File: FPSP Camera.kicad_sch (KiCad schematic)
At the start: 0 parts

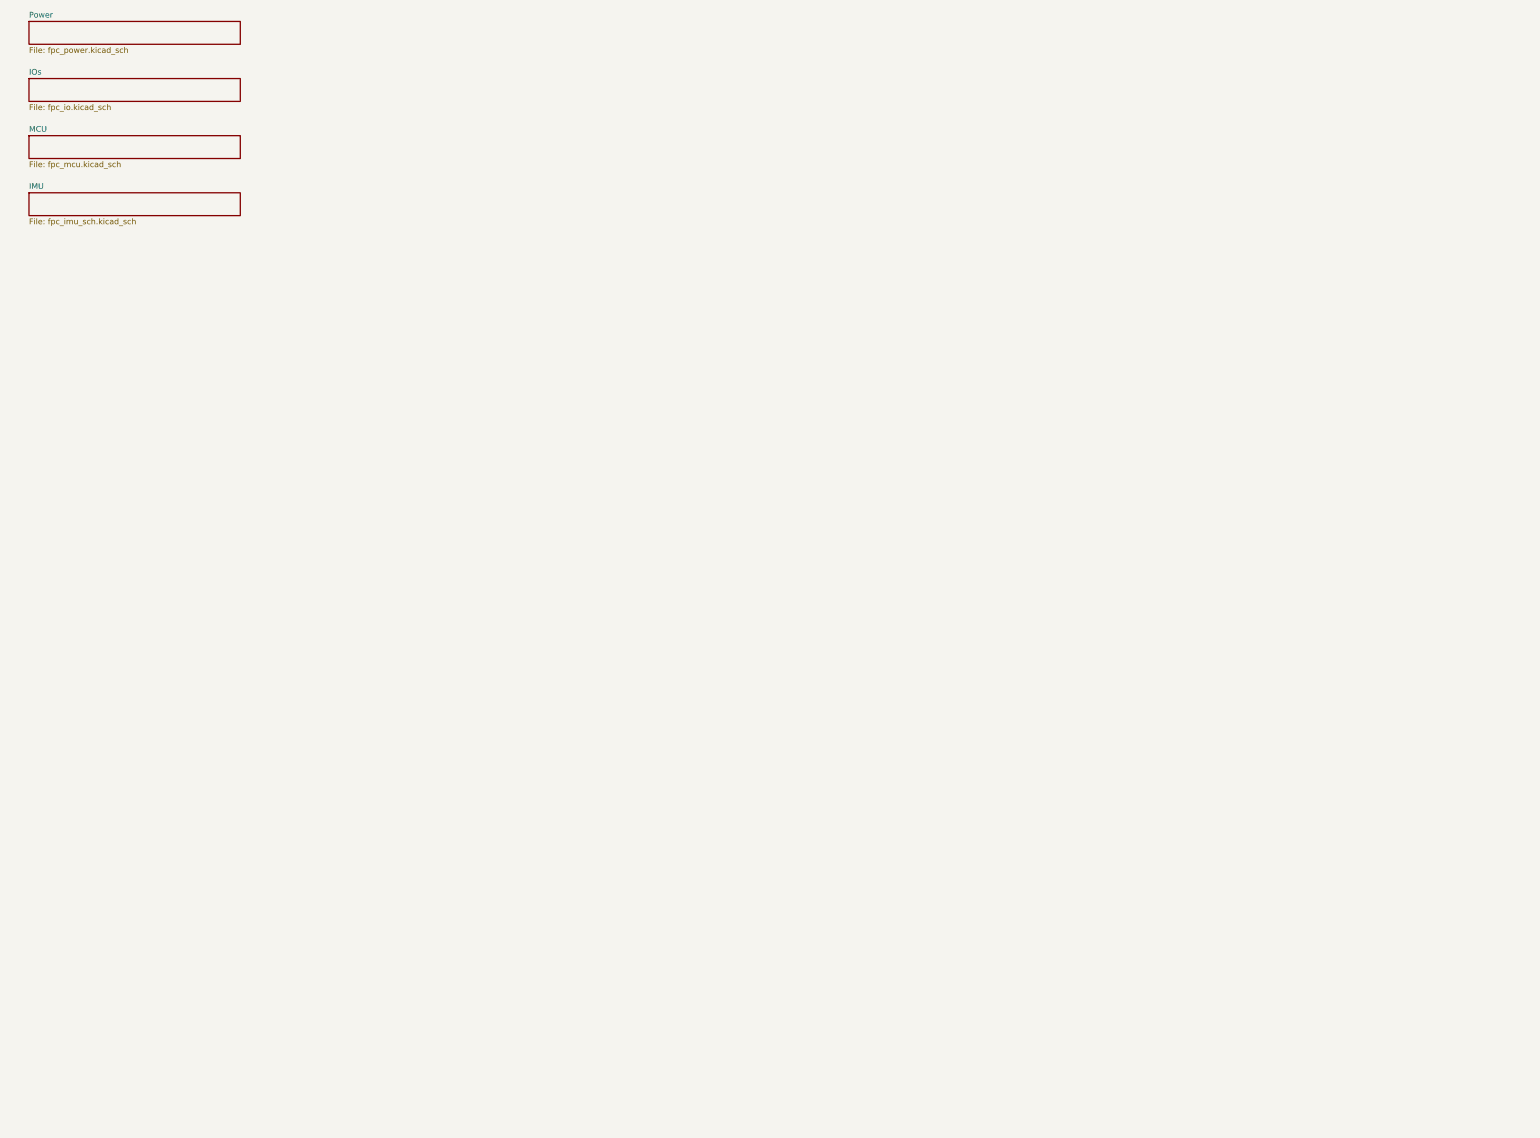
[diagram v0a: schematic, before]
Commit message: Cleanup
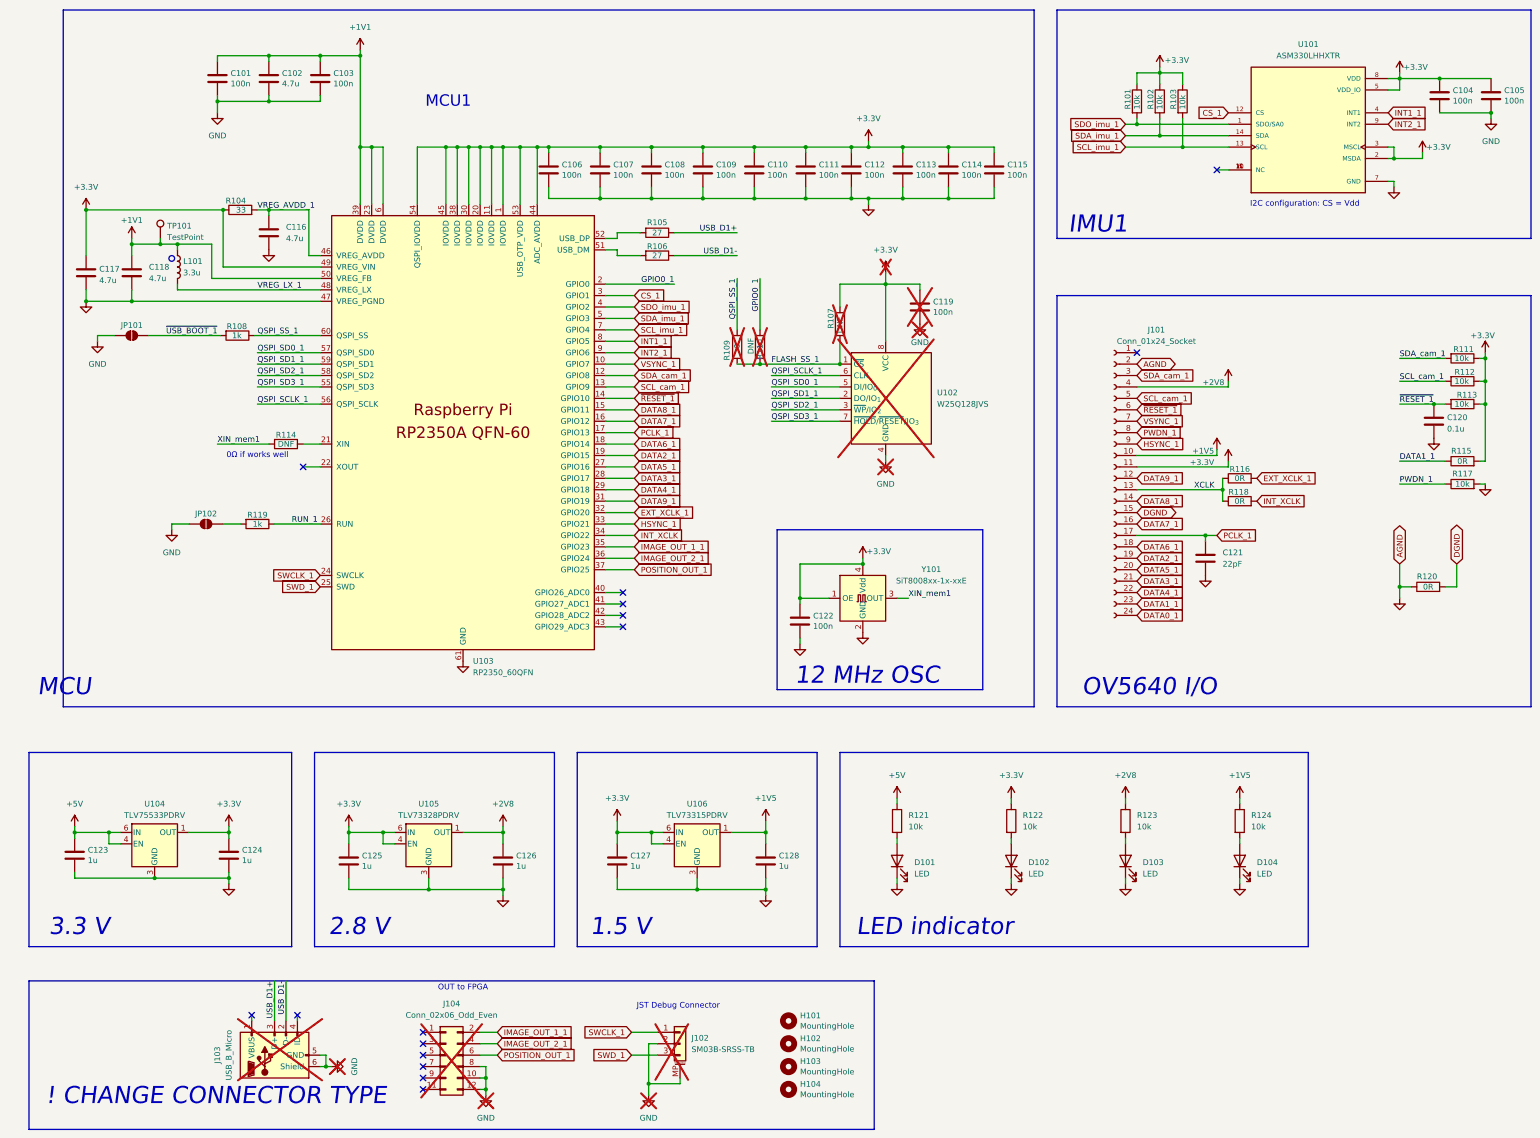
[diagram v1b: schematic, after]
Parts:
- added C101, C103, C104, C105, C106, C107, C108, C109, C110, C111, C112, C113, C114, C115, C119, C122: 100n, Capacitor_SMD:C_0603_1608Metric_Pad1.08x0.95mm_HandSolder, symbol Device:C
- added C102, C116, C117, C118: 4.7u, Capacitor_SMD:C_0603_1608Metric_Pad1.08x0.95mm_HandSolder, symbol Device:C
- added C120: 0.1u, Capacitor_SMD:C_0603_1608Metric_Pad1.08x0.95mm_HandSolder, symbol Device:C
- added C121: 22pF, Capacitor_SMD:C_0603_1608Metric_Pad1.08x0.95mm_HandSolder, symbol Device:C
- added C123, C124, C125, C126, C127, C128: 1u, Capacitor_SMD:C_0603_1608Metric_Pad1.08x0.95mm_HandSolder, symbol Device:C
- added D101, D102, D103, D104: LED, Diode_SMD:D_0603_1608Metric, symbol Device:LED
- added H101, H102, H103, H104: MountingHole, MountingHole:MountingHole_2.7mm_M2.5, symbol Mechanical:MountingHole
- added J101: Conn_01x24_Socket, Connector_FFC-FPC:TE_2-84952-4_1x24-1MP_P1.0mm_Horizontal, symbol Connector:Conn_01x24_Socket
- added J102: SM03B-SRSS-TB, Connector_JST:JST_SH_SM03B-SRSS-TB_1x03-1MP_P1.00mm_Horizontal, symbol Connector_Generic_MountingPin:Conn_01x03_MountingPin
- added J103: USB_B_Micro, RP2350_60QFN_minimal:USB_Micro-B_Amphenol_10103594-0001LF_Horizontal_modified, symbol Connector:USB_B_Micro
- added J104: Conn_02x06_Odd_Even, Connector_PinHeader_2.54mm:PinHeader_2x06_P2.54mm_Vertical, symbol Connector_Generic:Conn_02x06_Odd_Even
- added JP101, JP102: SolderJumper_2_Open, Jumper:SolderJumper-2_P1.3mm_Open_RoundedPad1.0x1.5mm, symbol Jumper:SolderJumper_2_Open
- added L101: 3.3u, Inductor_SMD:L_1210_3225Metric, symbol Device:L
- added R101, R102, R103, R111, R112, R113, R117, R121, R122, R123, R124: 10k, Resistor_SMD:R_0603_1608Metric_Pad0.98x0.95mm_HandSolder, symbol Device:R
- added R104: 33, Resistor_SMD:R_0603_1608Metric_Pad0.98x0.95mm_HandSolder, symbol Device:R
- added R105, R106: 27, Resistor_SMD:R_0603_1608Metric_Pad0.98x0.95mm_HandSolder, symbol Device:R
- added R107, R110, R114: DNF, Resistor_SMD:R_0603_1608Metric_Pad0.98x0.95mm_HandSolder, symbol Device:R
- added R108, R119: 1k, Resistor_SMD:R_0603_1608Metric_Pad0.98x0.95mm_HandSolder, symbol Device:R
- added R109: 0, Resistor_SMD:R_0603_1608Metric_Pad0.98x0.95mm_HandSolder, symbol Device:R
- added R115, R116, R118, R120: 0R, Resistor_SMD:R_0603_1608Metric_Pad0.98x0.95mm_HandSolder, symbol Device:R
- added TP101: TestPoint, TestPoint:TestPoint_Pad_D1.0mm, symbol Connector:TestPoint
- added U101: ASM330LHHXTR, ASM330LHHXTR:XDCR_ASM330LHHXTR, symbol ASM330LHHXTR:ASM330LHHXTR
- added U102: W25Q128JVS, Package_SO:SOIC-8_5.3x5.3mm_P1.27mm, symbol Memory_Flash:W25Q128JVS
- added U103: RP2350_60QFN, projLib:RP2350-QFN-60-1EP_7x7_P0.4mm_EP3.4x3.4mm_ThermalVias, symbol MCU_RaspberryPi_RP2350:RP2350_60QFN
- added U104: TLV75533PDRV, Package_SON:WSON-6-1EP_2x2mm_P0.65mm_EP1x1.6mm, symbol Regulator_Linear:TLV75533PDRV
- added U105: TLV73328PDRV, Package_SON:WSON-6-1EP_2x2mm_P0.65mm_EP1x1.6mm, symbol Regulator_Linear:TLV75533PDRV
- added U106: TLV73315PDRV, Package_SON:WSON-6-1EP_2x2mm_P0.65mm_EP1x1.6mm, symbol Regulator_Linear:TLV75533PDRV
- added Y101: SiT8008xx-1x-xxE, Oscillator:Oscillator_SMD_SiT_PQFN-4Pin_2.5x2.0mm, symbol Oscillator:SiT8008xx-1x-xxE
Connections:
- new net: R105.2, U103.52 (USB_DP)
- new net: R106.2, U103.51 (USB_DM)
- new net: JP102.2 (B), R119.2
- new net: R114.1, U103.21 (XIN)
- new net: D103.2 (A), R123.2
- new net: D102.2 (A), R122.2
- new net: D104.2 (A), R124.2
- new net: D101.2 (A), R121.2
- new net: U101.10 (NC), U101.11 (NC), U101.6 (NC)
- new net +1V1: C101.1, C102.1, C103.1, C118.1, L101.1, TP101.1, U103.23 (DVDD), U103.39 (DVDD), U103.50 (VREG_FB), U103.6 (DVDD)
- new net +1V5: C128.1, J101.10 (Pin_10), R124.1, U106.1 (OUT)
- new net +2V8: C126.1, J101.4 (Pin_4), R123.1, U105.1 (OUT)
- new net +3.3V: C104.1, C105.1, C106.1, C107.1, C108.1, C109.1, C110.1, C111.1, C112.1, C113.1, C114.1, C115.1, C117.1, C119.1, C122.1, C124.1, C125.1, C127.1, J101.11 (Pin_11), R101.1, R102.1, R103.1, R104.1, R107.1, R111.1, R112.1, R113.1, R115.2, R122.1, U101.2 (MSDA), U101.3 (MSCL), U101.5 (VDD_IO), U101.8 (VDD), U102.8 (VCC), U103.1 (IOVDD), U103.11 (IOVDD), U103.20 (IOVDD), U103.30 (IOVDD), U103.38 (IOVDD), U103.44 (ADC_AVDD), U103.45 (IOVDD), U103.49 (VREG_VIN), U103.53 (USB_OTP_VDD), U103.54 (QSPI_IOVDD), U104.1 (OUT), U105.4 (EN), U105.6 (IN), U106.4 (EN), U106.6 (IN), Y101.1 (OE), Y101.4 (Vdd)
- new net +5V: C123.1, R121.1, U104.4 (EN), U104.6 (IN)
- new net CS_1: U101.12 (CS), U103.3 (GPIO1)
- new net DATA0_1: J101.24 (Pin_24)
- new net DATA1_1: J101.23 (Pin_23), R115.1
- new net DATA2_1: J101.19 (Pin_19), U103.19 (GPIO15)
- new net DATA3_1: J101.21 (Pin_21), U103.28 (GPIO17)
- new net DATA4_1: J101.22 (Pin_22), U103.29 (GPIO18)
- new net DATA5_1: J101.20 (Pin_20), U103.27 (GPIO16)
- new net DATA6_1: J101.18 (Pin_18), U103.18 (GPIO14)
- new net DATA7_1: J101.16 (Pin_16), U103.16 (GPIO12)
- new net DATA8_1: J101.14 (Pin_14), U103.15 (GPIO11)
- new net DATA9_1: J101.12 (Pin_12), U103.31 (GPIO19)
- new net DGND: J101.15 (Pin_15), R120.2
- new net EXT_XCLK_1: R116.2, U103.32 (GPIO20)
- new net FLASH_SS_1: R107.2, R109.1, R110.1, U102.1 (~{CS})
- new net GND: C101.2, C102.2, C103.2, C104.2, C105.2, C106.2, C107.2, C108.2, C109.2, C110.2, C111.2, C112.2, C113.2, C114.2, C115.2, C116.2, C117.2, C118.2, C119.2, C120.2, C121.2, C122.2, C123.2, C124.2, C125.2, C126.2, C127.2, C128.2, D101.1 (K), D102.1 (K), D103.1 (K), D104.1 (K), J101.2 (Pin_2), J102.2 (Pin_2), J102.MP (MountPin), J103.5 (GND), J103.6 (Shield), J104.10 (Pin_10), J104.12 (Pin_12), J104.8 (Pin_8), JP101.1 (A), JP102.1 (A), R117.2, R120.1, U101.7 (GND), U102.4 (GND), U103.47 (VREG_PGND), U103.61 (GND), U104.3 (GND), U104.7 (GND), U105.3 (GND), U105.7 (GND), U106.3 (GND), U106.7 (GND), Y101.2 (GND)
- new net GPIO0_1: R110.2, U103.2 (GPIO0)
- new net HSYNC_1: J101.9 (Pin_9), U103.33 (GPIO21)
- new net IMAGE_OUT_1_1: J104.2 (Pin_2), U103.35 (GPIO23)
- new net IMAGE_OUT_2_1: J104.4 (Pin_4), U103.36 (GPIO24)
- new net INT1_1: U101.4 (INT1), U103.8 (GPIO5)
- new net INT2_1: U101.9 (INT2), U103.9 (GPIO6)
- new net INT_XCLK: R118.2, U103.34 (GPIO22)
- new net PCLK_1: C121.1, J101.17 (Pin_17), U103.17 (GPIO13)
- new net POSITION_OUT_1: J104.6 (Pin_6), U103.37 (GPIO25)
- new net PWDN_1: J101.8 (Pin_8), R117.1
- new net QSPI_SCLK_1: U102.6 (CLK), U103.56 (QSPI_SCLK)
- new net QSPI_SD0_1: U102.5 (DI/IO_{0}), U103.57 (QSPI_SD0)
- new net QSPI_SD1_1: U102.2 (DO/IO_{1}), U103.59 (QSPI_SD1)
- new net QSPI_SD2_1: U102.3 (~{WP}/IO_{2}), U103.58 (QSPI_SD2)
- new net QSPI_SD3_1: U102.7 (~{HOLD}/~{RESET}/IO_{3}), U103.55 (QSPI_SD3)
- new net QSPI_SS_1: R108.1, R109.2, U103.60 (QSPI_SS)
- new net RUN_1: R119.1, U103.26 (RUN)
- new net SCL_cam_1: J101.5 (Pin_5), R112.2, U103.13 (GPIO9)
- new net SCL_imu_1: R103.2, U101.13 (SCL), U103.7 (GPIO4)
- new net SDA_cam_1: J101.3 (Pin_3), R111.2, U103.12 (GPIO8)
- new net SDA_imu_1: R102.2, U101.14 (SDA), U103.5 (GPIO3)
- new net SDO_imu_1: R101.2, U101.1 (SDO/SA0), U103.4 (GPIO2)
- new net SWCLK_1: J102.1 (Pin_1), U103.24 (SWCLK)
- new net SWD_1: J102.3 (Pin_3), U103.25 (SWD)
- new net USB_D1+: J103.3 (D+), R105.1
- new net USB_D1-: J103.2 (D-), R106.1
- new net VREG_AVDD_1: C116.1, R104.2, U103.46 (VREG_AVDD)
- new net VREG_LX_1: L101.2, U103.48 (VREG_LX)
- new net VSYNC_1: J101.7 (Pin_7), U103.10 (GPIO7)
- new net XCLK: J101.13 (Pin_13), R116.1, R118.1
- new net XIN_mem1: R114.2, Y101.3 (OUT)
- new net ~{RESET_1}: C120.1, J101.6 (Pin_6), R113.2, U103.14 (GPIO10)
- new net ~{USB_BOOT_1}: JP101.2 (B), R108.2
- no-connect marks 0 -> 15
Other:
- removed sheet IMU
- removed sheet IOs
- removed sheet MCU
- removed sheet Power
- note added: "! CHANGE CONNECTOR TYPE"
- note added: "0Ω if works well"
- note added: "1.5 V"
- note added: "12 MHz OSC"
- note added: "2.8 V"
- note added: "3.3 V"
- note added: "I2C configuration: CS = Vdd"
- note added: "IMU1"
- note added: "JST Debug Connector"
- note added: "LED indicator"
- note added: "MCU"
- note added: "MCU1"
- note added: "OUT to FPGA"
- note added: "OV5640 I/O"
